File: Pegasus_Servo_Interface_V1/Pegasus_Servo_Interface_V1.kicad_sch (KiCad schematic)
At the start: 16 parts, among them J1 RJ45, J2 Pos_Feedback, J3 DE9_Receptacle_MountingHoles, U1 XC6216D332PR-G, U2 SN65LVDS2D

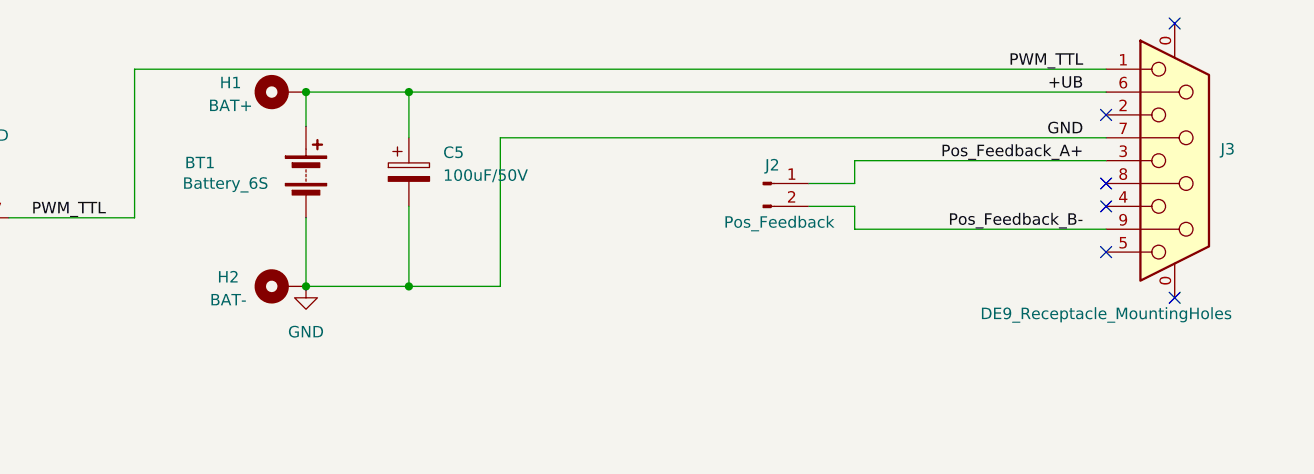
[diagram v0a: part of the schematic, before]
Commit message: Add files via upload
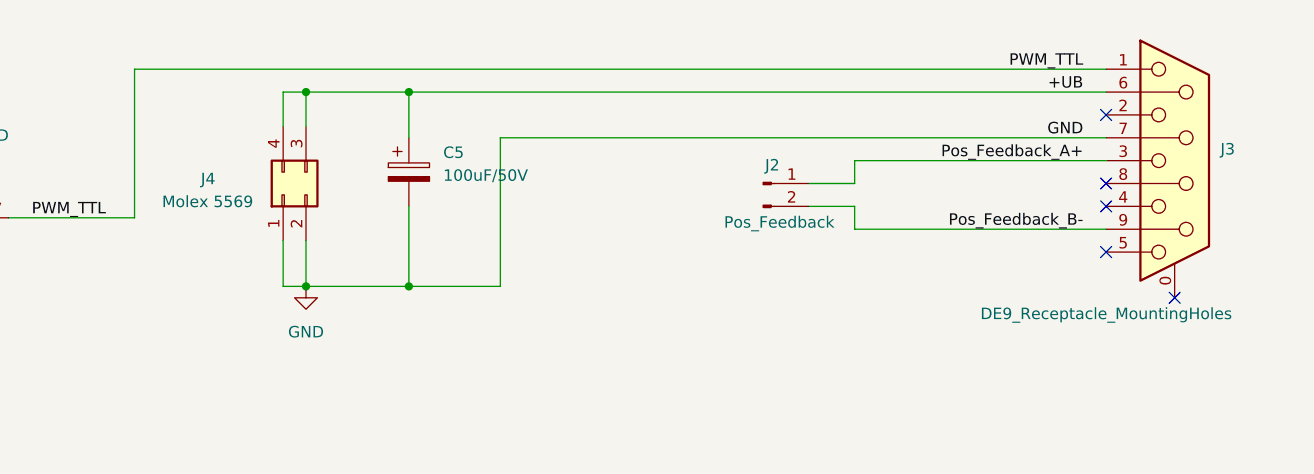
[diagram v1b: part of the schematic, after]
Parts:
- removed BT1: Battery_6S, symbol Device:Battery
- removed H1: BAT+, MountingHole:MountingHole_3.2mm_M3_DIN965_Pad_TopBottom, symbol Mechanical:MountingHole_Pad
- removed H2: BAT-, MountingHole:MountingHole_3.2mm_M3_DIN965_Pad_TopBottom, symbol Mechanical:MountingHole_Pad
- added J4: Molex 5569, Connector_Molex:Molex_Mini-Fit_Jr_5569-04A2_2x02_P4.20mm_Horizontal, symbol Connector_Generic:Conn_02x02_Counter_Clockwise
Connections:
- net +UB: now also J4.3 (Pin_3), J4.4 (Pin_4)
- net GND: now also J4.1 (Pin_1), J4.2 (Pin_2)
- no-connect marks 10 -> 9
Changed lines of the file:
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@@
+	)
+	(junction
+		(at 160.02 36.83)
+		(diameter 0)
+		(color 0 0 0 0)
 	)
 	(junction
@@
 	)
 	(junction
-		(at 160.02 36.83)
-		(diameter 0)
-		(color 0 0 0 0)
-	)
-	(junction
 		(at 104.14 35.56)
 		(diameter 0)
@@
 	)
 	(no_connect
-		(at 256.54 29.21)
-	)
-	(no_connect
 		(at 119.38 60.96)
 	)
@@
 	(wire
 		(pts
+			(xy 157.48 40.64) (xy 157.48 36.83)
+		)
+		(stroke
+			(width 0)
+			(type default)
+		)
+	)
+	(wire
+		(pts
 			(xy 104.14 41.91) (xy 104.14 40.64)
 		)
@@
 	(wire
 		(pts
+			(xy 157.48 36.83) (xy 160.02 36.83)
+		)
+		(stroke
+			(width 0)
+			(type default)
+		)
+	)
+	(wire
+		(pts
 			(xy 88.9 91.44) (xy 88.9 92.71)
 		)
@@
 	(wire
 		(pts
+			(xy 157.48 53.34) (xy 157.48 58.42)
+		)
+		(stroke
+			(width 0)
+			(type default)
+		)
+	)
+	(wire
+		(pts
 			(xy 95.25 53.34) (xy 101.6 53.34)
 		)
@@
 	(wire
 		(pts
+			(xy 160.02 53.34) (xy 160.02 58.42)
+		)
+		(stroke
+			(width 0)
+			(type default)
+		)
+	)
+	(wire
+		(pts
 			(xy 220.98 44.45) (xy 220.98 46.99)
 		)
@@
 	(wire
 		(pts
-			(xy 160.02 50.8) (xy 160.02 58.42)
-		)
-		(stroke
-			(width 0)
-			(type default)
-		)
-	)
-	(wire
-		(pts
 			(xy 43.18 107.95) (xy 67.31 107.95)
 		)
@@
 		(pts
 			(xy 104.14 35.56) (xy 114.3 35.56)
+		)
+		(stroke
+			(width 0)
+			(type default)
+		)
+	)
+	(wire
+		(pts
+			(xy 157.48 58.42) (xy 160.02 58.42)
 		)
 		(stroke
@@
 	)
 	(symbol
+		(lib_id "Connector_Generic:Conn_02x02_Counter_Clockwise")
+		(at 157.48 48.26 90)
+		(unit 1)
+		(exclude_from_sim no)
+		(in_bom yes)
+		(on_board yes)
+		(dnp no)
+		(property "Reference" "J4"
+			(at 148.336 46.482 90)
+			(effects
+				(font
+					(size 1.27 1.27)
+				)
+				(justify right)
+			)
+		)
+		(property "Value" "Molex 5569"
+			(at 144.018 49.022 90)
+			(effects
+				(font
+					(size 1.27 1.27)
+				)
+				(justify right)
+			)
+		)
+		(property "Footprint" "Connector_Molex:Molex_Mini-Fit_Jr_5569-04A2_2x02_P4.20mm_Horizontal"
+			(at 157.48 48.26 0)
+			(effects
+				(font
+					(size 1.27 1.27)
+				)
+				(hide yes)
+			)
+		)
+		(property "Datasheet" "https://www.molex.com/en-us/products/part-detail/26013115?display=pdf "
+			(at 157.48 48.26 0)
+			(effects
+				(font
+					(size 1.27 1.27)
+				)
+				(hide yes)
+			)
+		)
+		(property "Description" "Generic connector, double row, 02x02, counter clockwise pin numbering scheme (similar to DIP package numbering), script generated (kicad-library-utils/schlib/autogen/connector/)"
+			(at 157.48 48.26 0)
+			(effects
+				(font
+					(size 1.27 1.27)
+				)
+				(hide yes)
+			)
+		)
+		(property "Link" "https://www.digikey.jp/en/products/detail/molex/0026013115/4119889"
+			(at 157.48 48.26 0)
+			(effects
+				(font
+					(size 1.27 1.27)
+				)
+				(hide yes)
+			)
+		)
+		(property "MPN" "0026013115"
+			(at 157.48 48.26 0)
+			(effects
+				(font
+					(size 1.27 1.27)
+				)
+				(hide yes)
+			)
+		)
+		(pin "4"
+		)
+		(pin "2"
+		)
+		(pin "3"
+		)
+		(pin "1"
+		)
+		(instances
+			(project ""
+				(path "/33d08739-9df2-4e53-9b99-51d634eccd8e"
+					(reference "J4")
+					(unit 1)
+				)
+			)
+		)
+	)
+	(symbol
 		(lib_id "power:GND")
 		(at 95.25 41.91 0)
@@
 	)
 	(symbol
-		(lib_id "Mechanical:MountingHole_Pad")
-		(at 157.48 58.42 90)
-		(unit 1)
-		(exclude_from_sim yes)
-		(in_bom no)
-		(on_board yes)
-		(dnp no)
-		(property "Reference" "H2"
-			(at 151.384 57.404 90)
-			(effects
-				(font
-					(size 1.27 1.27)
-				)
-			)
-		)
-		(property "Value" "BAT-"
-			(at 151.384 59.944 90)
-			(effects
-				(font
-					(size 1.27 1.27)
-				)
-			)
-		)
-		(property "Footprint" "MountingHole:MountingHole_3.2mm_M3_DIN965_Pad_TopBottom"
-			(at 157.48 58.42 0)
-			(effects
-				(font
-					(size 1.27 1.27)
-				)
-				(hide yes)
-			)
-		)
-		(property "Datasheet" "~"
-			(at 157.48 58.42 0)
-			(effects
-				(font
-					(size 1.27 1.27)
-				)
-				(hide yes)
-			)
-		)
-		(property "Description" "Mounting Hole with connection"
-			(at 157.48 58.42 0)
-			(effects
-				(font
-					(size 1.27 1.27)
-				)
-				(hide yes)
-			)
-		)
-		(pin "1"
-		)
-		(instances
-			(project ""
-				(path "/33d08739-9df2-4e53-9b99-51d634eccd8e"
-					(reference "H2")
-					(unit 1)
-				)
-			)
-		)
-	)
-	(symbol
 		(lib_id "Connector:RJ45_Shielded")
 		(at 49.53 55.88 0)
@@
 				(path "/33d08739-9df2-4e53-9b99-51d634eccd8e"
 					(reference "C3")
-					(unit 1)
-				)
-			)
-		)
-	)
-	(symbol
-		(lib_id "Device:Battery")
-		(at 160.02 45.72 0)
-		(unit 1)
-		(exclude_from_sim no)
-		(in_bom no)
-		(on_board no)
-		(dnp no)
-		(property "Reference" "BT1"
-			(at 146.558 44.704 0)
-			(effects
-				(font
-					(size 1.27 1.27)
-				)
-				(justify left)
-			)
-		)
-		(property "Value" "Battery_6S"
-			(at 146.304 46.99 0)
-			(effects
-				(font
-					(size 1.27 1.27)
-				)
-				(justify left)
-			)
-		)
-		(property "Footprint" ""
-			(at 160.02 44.196 90)
-			(effects
-				(font
-					(size 1.27 1.27)
-				)
-				(hide yes)
-			)
-		)
-		(property "Datasheet" "~"
-			(at 160.02 44.196 90)
-			(effects
-				(font
-					(size 1.27 1.27)
-				)
-				(hide yes)
-			)
-		)
-		(property "Description" "Multiple-cell battery"
-			(at 160.02 45.72 0)
-			(effects
-				(font
-					(size 1.27 1.27)
-				)
-				(hide yes)
-			)
-		)
-		(pin "1"
-		)
-		(pin "2"
-		)
-		(instances
-			(project "Pegasus_Sensor_Interface"
-				(path "/33d08739-9df2-4e53-9b99-51d634eccd8e"
-					(reference "BT1")
 					(unit 1)
 				)
@@
 	)
 	(symbol
-		(lib_id "Mechanical:MountingHole_Pad")
-		(at 157.48 36.83 90)
-		(unit 1)
-		(exclude_from_sim yes)
-		(in_bom no)
-		(on_board yes)
-		(dnp no)
-		(property "Reference" "H1"
-			(at 151.638 35.814 90)
-			(effects
-				(font
-					(size 1.27 1.27)
-				)
-			)
-		)
-		(property "Value" "BAT+"
-			(at 151.638 38.354 90)
-			(effects
-				(font
-					(size 1.27 1.27)
-				)
-			)
-		)
-		(property "Footprint" "MountingHole:MountingHole_3.2mm_M3_DIN965_Pad_TopBottom"
-			(at 157.48 36.83 0)
-			(effects
-				(font
-					(size 1.27 1.27)
-				)
-				(hide yes)
-			)
-		)
-		(property "Datasheet" "~"
-			(at 157.48 36.83 0)
-			(effects
-				(font
-					(size 1.27 1.27)
-				)
-				(hide yes)
-			)
-		)
-		(property "Description" "Mounting Hole with connection"
-			(at 157.48 36.83 0)
-			(effects
-				(font
-					(size 1.27 1.27)
-				)
-				(hide yes)
-			)
-		)
-		(pin "1"
-		)
-		(instances
-			(project ""
-				(path "/33d08739-9df2-4e53-9b99-51d634eccd8e"
-					(reference "H1")
-					(unit 1)
-				)
-			)
-		)
-	)
-	(symbol
 		(lib_id "Connector:DE9_Receptacle_MountingHoles")
 		(at 256.54 44.45 0)
@@
 			)
 		)
-		(property "Datasheet" "https://www.assmann-wsw.com/uploads/datasheets/ASS_4888_CO.pdf"
+		(property "Datasheet" " ~"
 			(at 256.54 44.45 0)
 			(effects
@@
 		(pin "8"
 		)
-		(pin "0"
-		)
 		(instances
